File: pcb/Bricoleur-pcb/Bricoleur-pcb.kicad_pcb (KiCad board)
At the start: 2 copper layers, 68.6 x 124.5 mm, 78 parts, among them J1 USB_B_Micro, J2 Conn_02x10_Odd_Even, J3 Conn_02x03_Odd_Even, J4 Conn_02x03_Odd_Even, SW2 SW_Push, SW3 SW_Push, SW4 SW_Push, SW5 SW_Push, U1 Ultrasonic-LV-EZ0, U11 SW_DP3T, U2 PYNQ-Shield-Bricoleur-pcb-cac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, U3 Ultrasonic-LV-EZ0, U4 Ultrasonic-LV-EZ0, U5 Arducam-OV5642, U6 Arducam-OV5642, U7 EFM32GG980, U8 UART_BOOT, U9 IP4220CZ6, Y1 ABM2-48.000MHZ-D4YF-T

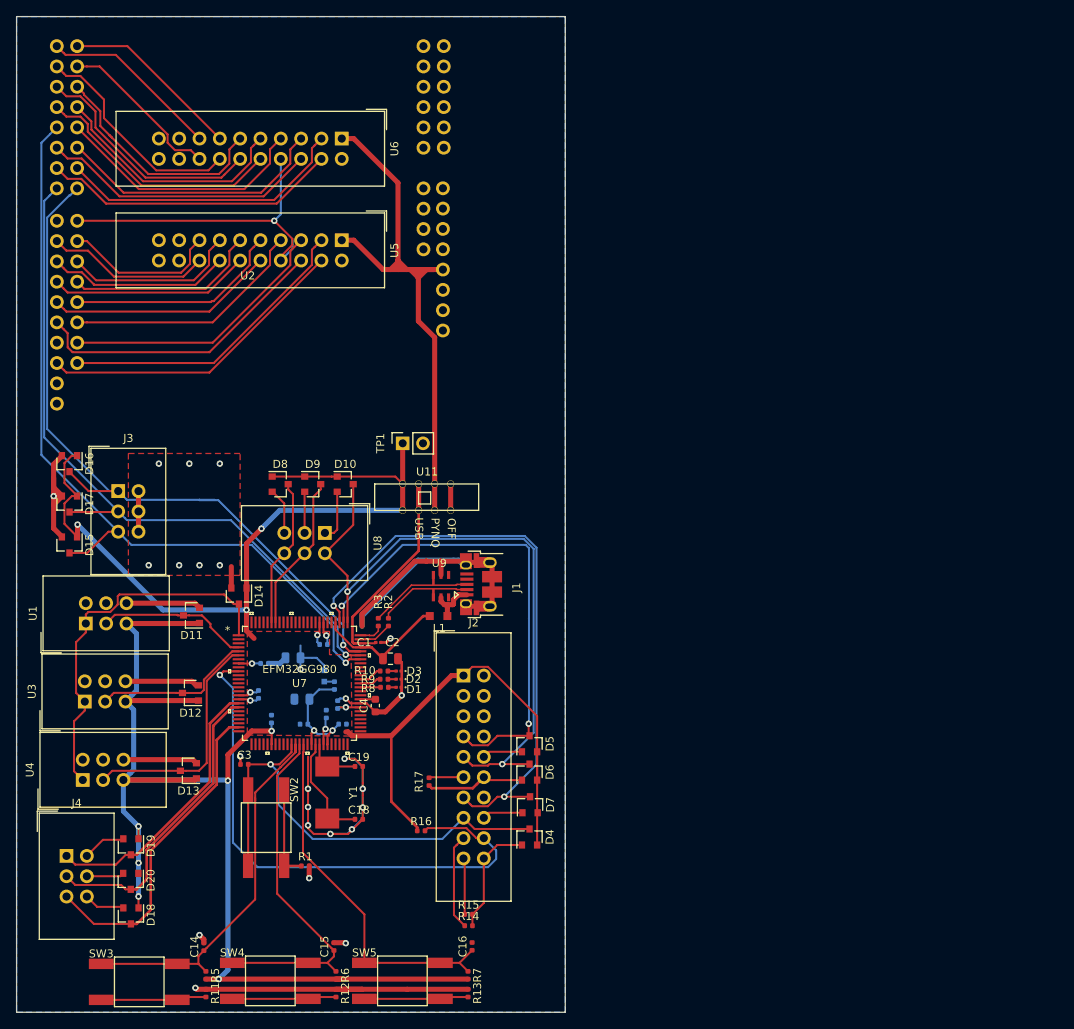
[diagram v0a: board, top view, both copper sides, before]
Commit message: Layout finished.
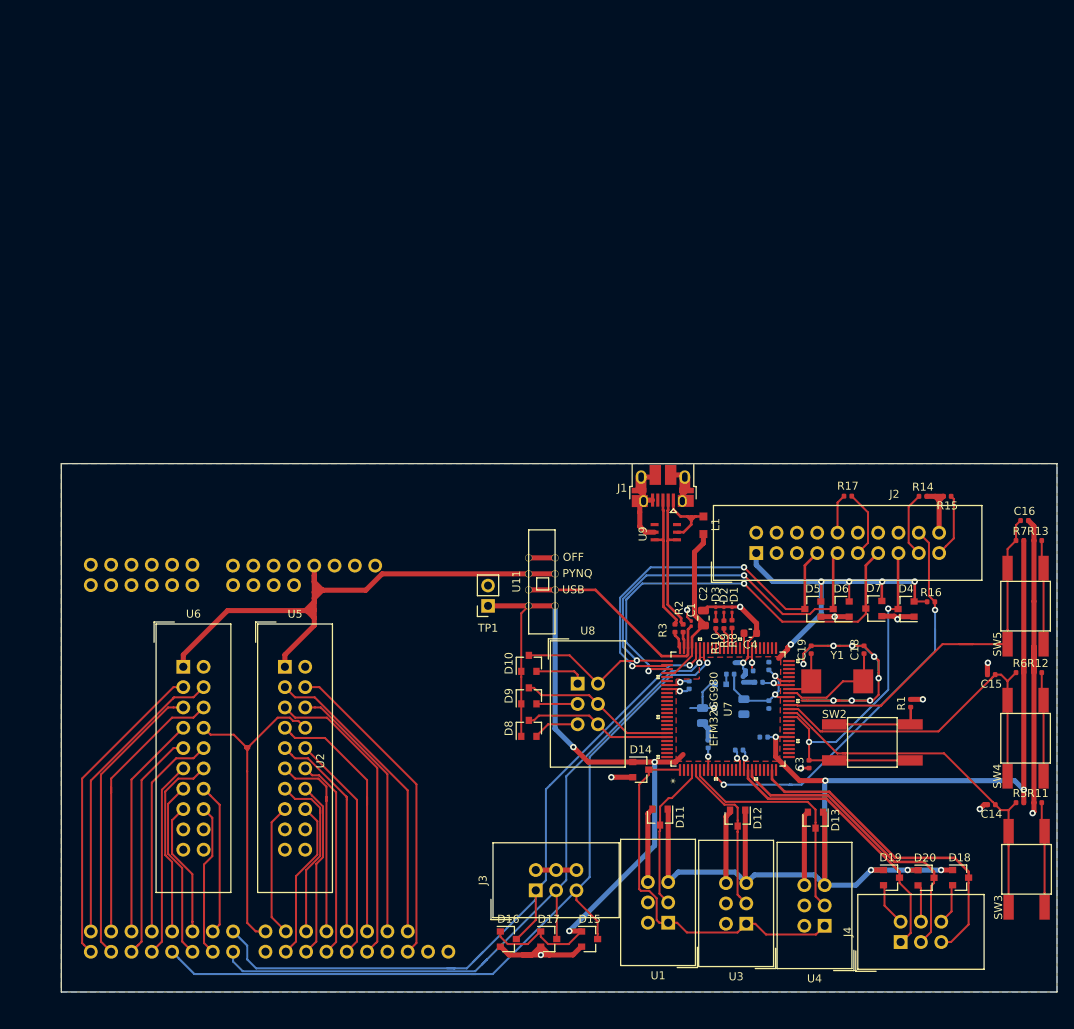
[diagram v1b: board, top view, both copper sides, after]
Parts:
- moved SW3 113.6 mm to (148.3, 158.3), turned to 90 degrees
- moved R11 106.7 mm to (152.0, 145.2), turned to 0 degrees
- moved J4 104.8 mm to (134.8, 162.6), turned to 90 degrees
- moved R5 104.0 mm to (149.7, 145.2), turned to 0 degrees
- moved D18 103.8 mm to (142.3, 154.6), turned to 0 degrees
- moved C14 100.0 mm to (146.2, 145.5), turned to 180 degrees
- moved SW4 99.7 mm to (148.2, 141.9), turned to 90 degrees
- moved D20 99.4 mm to (138.0, 154.6), turned to 0 degrees
- moved R12 96.5 mm to (152.0, 129.0), turned to 0 degrees
- moved D19 95.2 mm to (133.7, 154.6), turned to 0 degrees
- moved U4 94.5 mm to (125.3, 160.6), turned to 180 degrees
- moved R6 93.5 mm to (149.7, 129.0), turned to 0 degrees
- moved R13 91.0 mm to (152.0, 112.5), turned to 0 degrees
- moved SW5 89.7 mm to (148.2, 125.4), turned to 90 degrees
- moved C15 88.9 mm to (146.2, 129.2), turned to 180 degrees
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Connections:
- U2 pad 29: /CAM1_HREF -> /CAM1_VSYNC
- U2 pad 36: /CAM1_VSYNC -> /CAM1_HREF
- U2 pad 44: /CAM0_SDATA -> /CAM0_DOUT2
- U2 pad 45: /CAM0_HREF -> /CAM0_DOUT5
- U2 pad 47: /CAM0_DOUT8 -> /CAM0_DOUT7
- U2 pad 48: /CAM0_DOUT6 -> /CAM0_DOUT9
- U2 pad 49: /CAM0_DOUT4 -> /CAM0_VSYNC
- U2 pad 50: /CAM0_DOUT3 -> /CAM0_SCL
- U2 pad 52: /CAM0_SCL -> /CAM0_DOUT4
- U2 pad 53: /CAM0_VSYNC -> /CAM0_DOUT3
- U2 pad 54: /CAM0_PCLK -> /CAM0_DOUT6
- U2 pad 55: /CAM0_DOUT9 -> /CAM0_DOUT8
- U2 pad 56: /CAM0_DOUT7 -> /CAM0_PCLK
- U2 pad 57: /CAM0_DOUT2 -> /CAM0_HREF
- U2 pad 58: /CAM0_DOUT5 -> /CAM0_SDATA
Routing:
- net GND: track 286.8 -> 241.7 mm, vias 19 -> 22
- net DH_TDO_SWO: track 74.6 -> 54.3 mm
- net DH_TCK_SWCLK: track 83.7 -> 65.3 mm
- net DEBUG_EXT_CABLE_ATTACH: track 70.0 -> 53.3 mm, vias 1 -> 2
- net VMCU: track 342.9 -> 326.7 mm, vias 15 -> 20
- net DH_TMS_SWDIO: track 61.6 -> 48.0 mm
- net DH_#RESET: track 60.0 -> 50.7 mm, vias 1 -> 2
- net /CAM0_DOUT4: track 27.7 -> 19.0 mm
- net /CAM0_DOUT6: track 29.8 -> 23.8 mm
- net /CAM0_DOUT3: track 22.6 -> 16.9 mm
- net /USB_D-: track 12.7 -> 18.0 mm
- net /CAM0_DOUT7: track 29.4 -> 24.6 mm
- net /CAM0_DOUT8: track 31.5 -> 26.9 mm
- net /CAM1_HREF: track 37.9 -> 33.4 mm
- net /CAM0_PCLK: track 32.3 -> 28.1 mm
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- removed copper zone on F.Cu, net GND
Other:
- board size 68.6 x 124.5 mm -> 124.5 x 66 mm
- net class USB added: clearance 0, trace_width 0.254, via_dia 0.8, via_drill 0.4
